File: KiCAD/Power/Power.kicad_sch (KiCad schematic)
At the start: 18 parts, among them J1 Barrel_Jack_Switch_MountingPin, J2 Conn_01x03_Pin, U1 LM317L_SOT-89, U2 LM337_SOT223, U3 LM336Z-2.5v

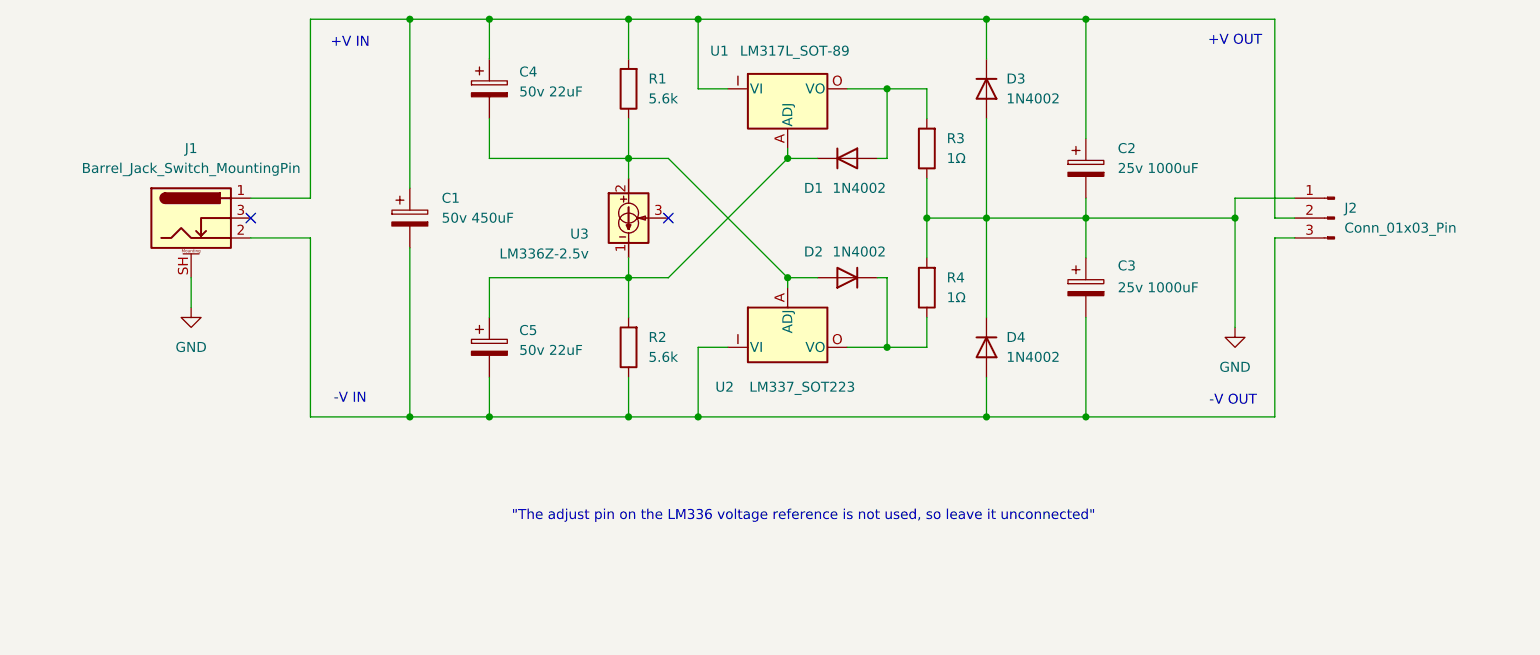
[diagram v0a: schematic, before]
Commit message: MidMount Capacitors
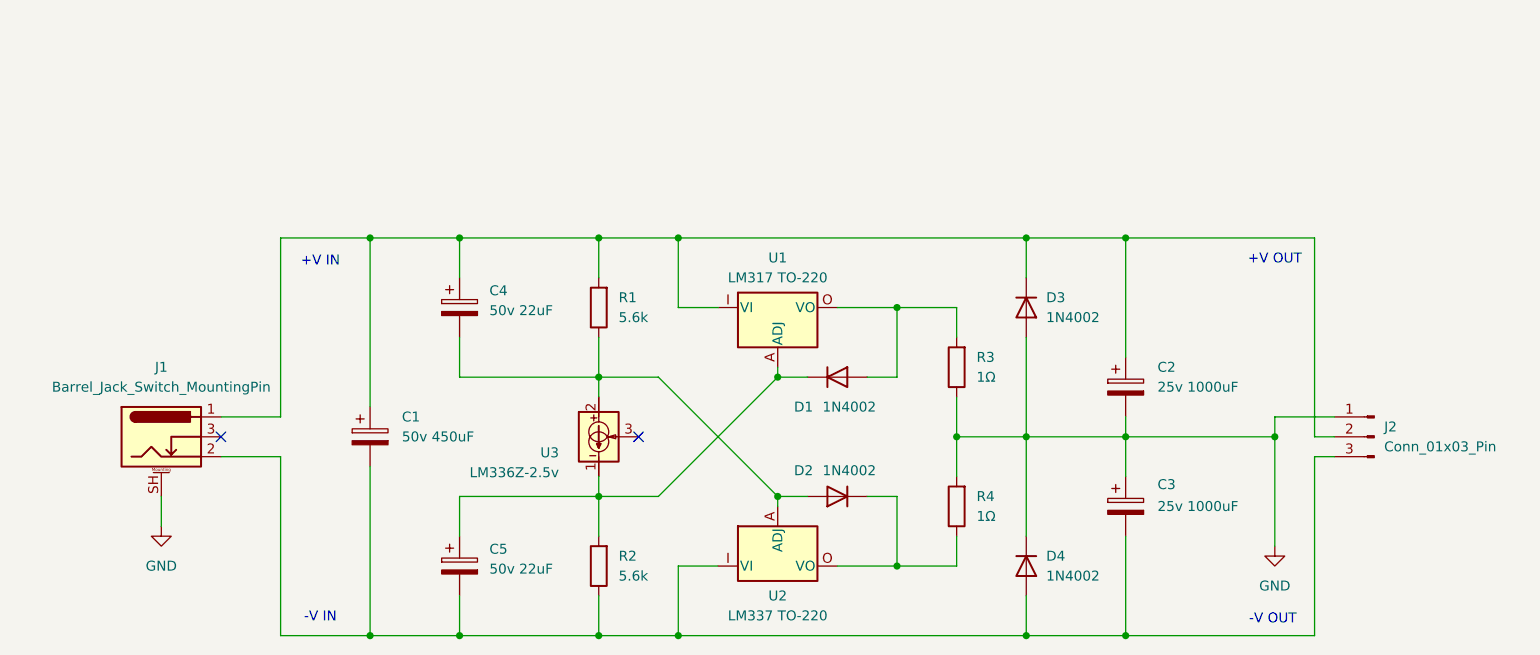
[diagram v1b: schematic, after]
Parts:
- removed U1: LM317L_SOT-89, HackSynth:LM317 - TO-220-3_Vertical, symbol Regulator_Linear:LM317L_SOT-89
- removed U2: LM337_SOT223, HackSynth:LM337 - TO-220-3_Vertical, symbol Regulator_Linear:LM337_SOT223
- added U1: LM317 TO-220, HackSynth:LM317 - TO-220-3_Horizontal_TabDown, symbol HackSynth:LM317 TO-220
- added U2: LM337 TO-220, HackSynth:LM337 - TO-220-3_Horizontal_TabDown, symbol HackSynth:LM337 TO-220
- C1, C2, C3: footprint Capacitor_THT:CP_Radial_D10.0mm_P5.00mm -> HackSynth:CP_Radial_D10.0mm_P5.00mm_MidMount
- U3: footprint HackSynth:TO-92_Inline - Handsolder -> Package_TO_SOT_THT:TO-92_Inline
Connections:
- net at D1.2 (A), R3.2: now also U1.O (VO)
- net at C1.2, C3.2, C5.2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: now also U2.I (VI)
- net at C4.2, D2.2 (A), R1.1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: now also U2.A (ADJ)
- net at C1.1, C2.1, C4.1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: now also U1.I (VI)
- net at D2.1 (K), R4.1: now also U2.O (VO)
- net at C5.1, D1.1 (K), R2.2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: now also U1.A (ADJ)
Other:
- note removed: ""The adjust pin on the LM336 voltage reference is not used, so leave it unconnected""
- moved on the sheet: C1, C2, C3, C4, C5, D1, D2, D3, D4, J1, J2, R1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

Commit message: Power PCB
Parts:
- U3: footprint Package_TO_SOT_THT:TO-92_Inline -> HackSynth:TO-92_Inline - Handsolder
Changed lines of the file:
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@@
 			)
 		)
-		(property "Footprint" "Package_TO_SOT_THT:TO-92_Inline"
+		(property "Footprint" "HackSynth:TO-92_Inline - Handsolder"
 			(at 120.015 89.535 0)
 			(effects
